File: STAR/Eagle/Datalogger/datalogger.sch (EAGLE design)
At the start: 6 parts, among them J1 J30J-25

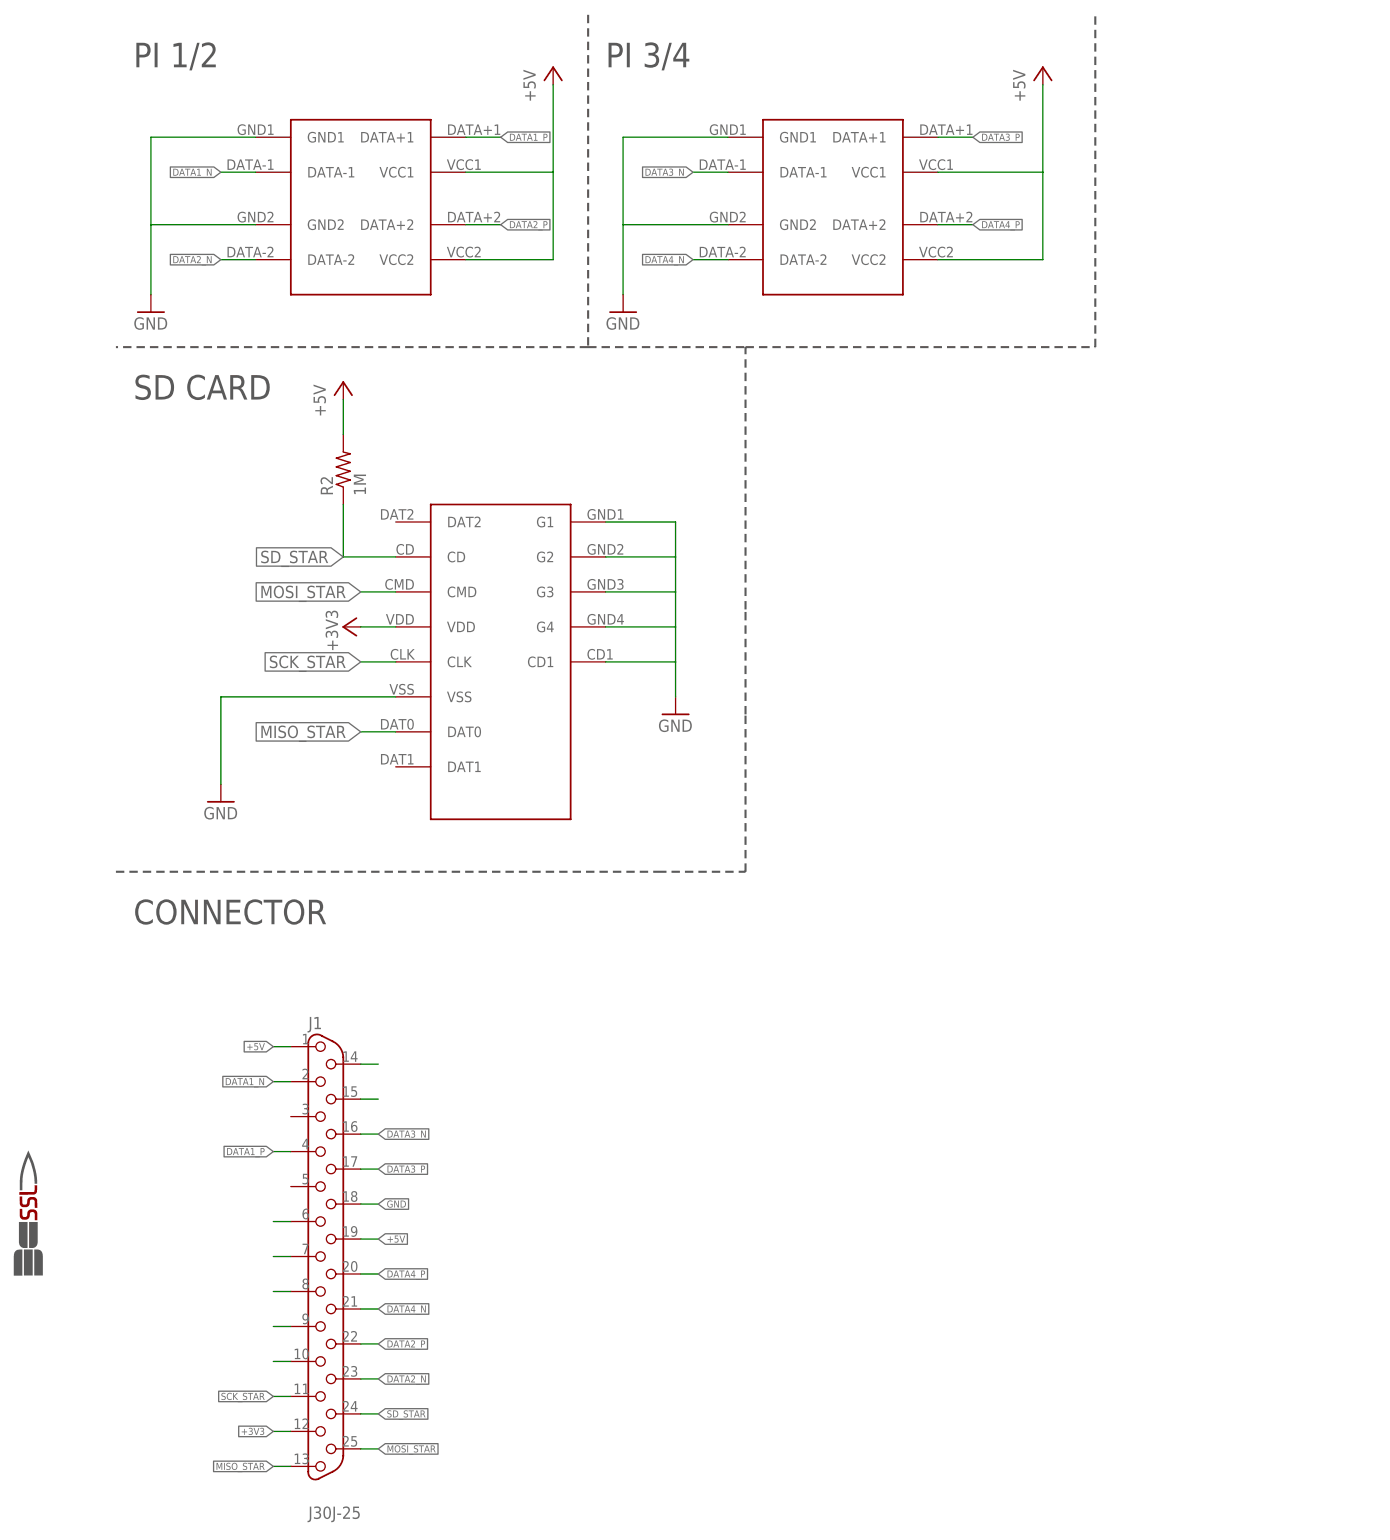
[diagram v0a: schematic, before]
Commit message: Datalogger v4
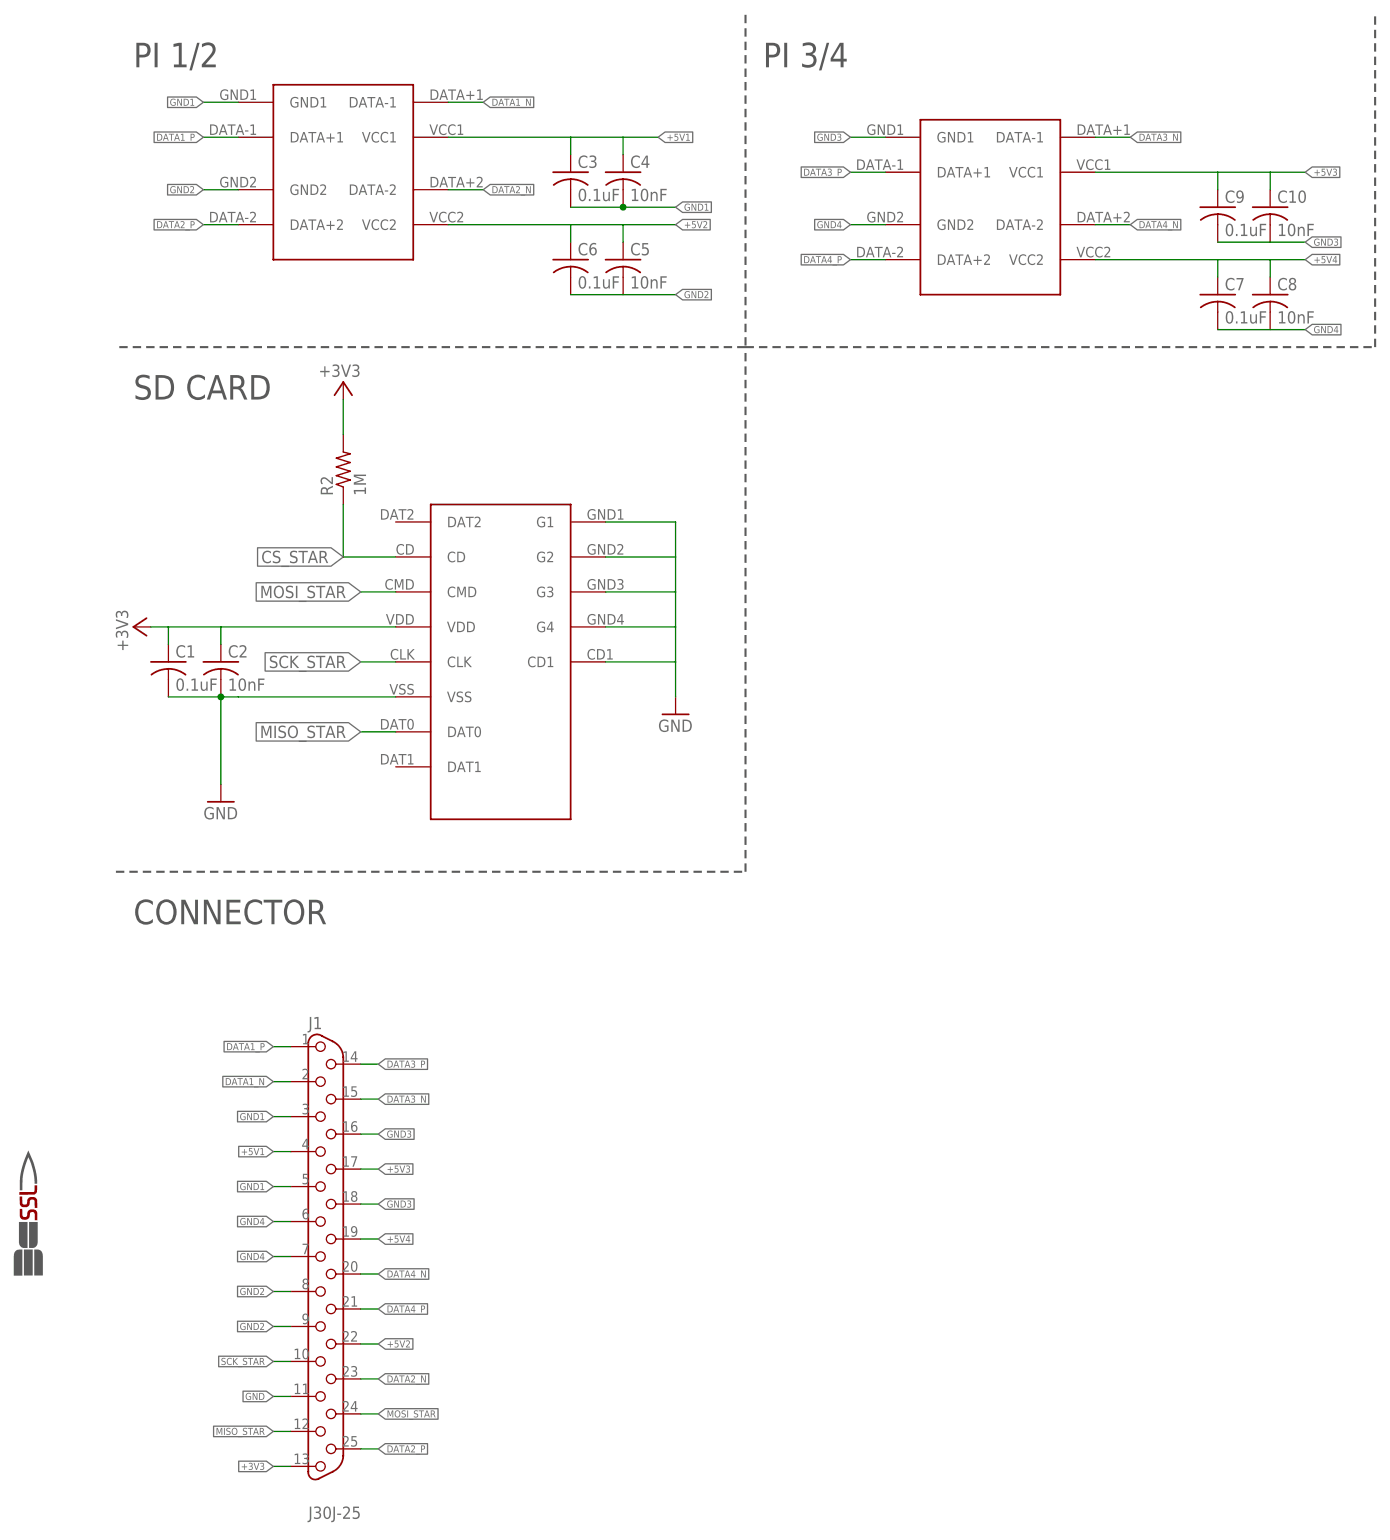
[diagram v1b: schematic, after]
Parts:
- added C1, C3, C6, C7, C9: 0.1uF, resistor:C-USC0603
- added C10, C2, C4, C5, C8: 10nF, resistor:C-USC0603
- renumbered U$4 to GND1
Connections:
- removed net +5V: J1.1, J1.19, R2.2, U$2.VCC1, U$2.VCC2, U$3.VCC1, U$3.VCC2
- removed net N$1: J1.14
- removed net N$2: J1.15
- removed net N$4: J1.6
- removed net N$5: J1.7
- removed net N$6: J1.8
- removed net N$7: J1.9
- removed net N$8: J1.10
- removed net SD_STAR: J1.24, R2.1, U$1.CD
- new net +5V1: C3.1, C4.1, J1.4, U$2.VCC1
- new net +5V2: C5.1, C6.1, J1.22, U$2.VCC2
- new net +5V3: C10.1, C9.1, J1.17, U$3.VCC1
- new net +5V4: C7.1, C8.1, J1.19, U$3.VCC2
- new net CS_STAR: R2.1, U$1.CD
- new net GND1: C3.2, C4.2, J1.3, J1.5, U$2.GND1
- new net GND2: C5.2, C6.2, J1.8, J1.9, U$2.GND2
- new net GND3: C10.2, C9.2, J1.16, J1.18, U$3.GND1
- new net GND4: C7.2, C8.2, J1.6, J1.7, U$3.GND2
- net +3V3: now also C1.1, C2.1, J1.13, R2.2; no longer J1.12
- net DATA1_P: now also J1.1; no longer J1.4
- net DATA2_P: now also J1.25; no longer J1.22
- net DATA3_N: now also J1.15; no longer J1.16
- net DATA3_P: now also J1.14; no longer J1.17
- net DATA4_N: now also J1.20; no longer J1.21
- net DATA4_P: now also J1.21; no longer J1.20
- net GND: now also C1.2, C2.2, J1.11; no longer J1.18, U$2.GND1, U$2.GND2, U$3.GND1, U$3.GND2
- net MISO_STAR: now also J1.12; no longer J1.13
- net MOSI_STAR: now also J1.24; no longer J1.25
- net SCK_STAR: now also J1.10; no longer J1.11
